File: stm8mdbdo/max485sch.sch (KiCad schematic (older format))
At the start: 1 part, among them U4 MAX485

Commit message: Решена проблемма с библиотекой для конденсаторов. Просто сделал копию папки с именем которое содержится в ошибке.
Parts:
- added R15, R16: 20K, symbol R
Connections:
- wire segments 8 -> 12
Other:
- note added: "Доделать: ставить терминатор, разъем."
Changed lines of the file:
@@
 LIBS:zetex
 LIBS:Zilog
+LIBS:rcl
 LIBS:stm8do-cache
 EELAYER 25 0
@@
 $EndComp
 $Comp
-L GND #PWR085
+L GND #PWR88
 U 1 1 5C686AB8
 P 5650 4600
-F 0 "#PWR085" H 5650 4350 50  0001 C CNN
+F 0 "#PWR88" H 5650 4350 50  0001 C CNN
 F 1 "GND" H 5650 4450 50  0000 C CNN
 F 2 "" H 5650 4600 50  0000 C CNN
@@
 	4650 4150 5050 4150
 $Comp
-L +5V #PWR086
+L +5V #PWR87
 U 1 1 5C6A210B
 P 5650 3250
-F 0 "#PWR086" H 5650 3100 50  0001 C CNN
+F 0 "#PWR87" H 5650 3100 50  0001 C CNN
 F 1 "+5V" H 5650 3390 50  0000 C CNN
 F 2 "" H 5650 3250 50  0000 C CNN
@@
 	4650 3900 4850 3900
 Connection ~ 4850 3900
+$Comp
+L R R15
+U 1 1 5C6B16A1
+P 8150 1850
+F 0 "R15" V 8230 1850 50  0000 C CNN
+F 1 "20K" V 8150 1850 50  0000 C CNN
+F 2 "" V 8080 1850 50  0000 C CNN
+F 3 "" H 8150 1850 50  0000 C CNN
+	1    8150 1850
+	1    0    0    -1
+$EndComp
+$Comp
+L R R16
+U 1 1 5C6B1766
+P 8850 1900
+F 0 "R16" V 8930 1900 50  0000 C CNN
+F 1 "20K" V 8850 1900 50  0000 C CNN
+F 2 "" V 8780 1900 50  0000 C CNN
+F 3 "" H 8850 1900 50  0000 C CNN
+	1    8850 1900
+	1    0    0    -1
+$EndComp
+$Comp
+L +5V #PWR89
+U 1 1 5C6B17A4
+P 8150 1700
+F 0 "#PWR89" H 8150 1550 50  0001 C CNN
+F 1 "+5V" H 8150 1840 50  0000 C CNN
+F 2 "" H 8150 1700 50  0000 C CNN
+F 3 "" H 8150 1700 50  0000 C CNN
+	1    8150 1700
+	1    0    0    -1
+$EndComp
+Text GLabel 8300 2200 2    60   Input ~ 0
+A
+Text GLabel 9000 1600 2    60   Input ~ 0
+B
+$Comp
+L GND #PWR90
+U 1 1 5C6B183A
+P 8850 2050
+F 0 "#PWR90" H 8850 1800 50  0001 C CNN
+F 1 "GND" H 8850 1900 50  0000 C CNN
+F 2 "" H 8850 2050 50  0000 C CNN
+F 3 "" H 8850 2050 50  0000 C CNN
+	1    8850 2050
+	1    0    0    -1
+$EndComp
+Wire Wire Line
+	8150 2000 8150 2200
+Wire Wire Line
+	8150 2200 8300 2200
+Wire Wire Line
+	9000 1600 8850 1600
+Wire Wire Line
+	8850 1600 8850 1750
+Text Notes 4400 1250 0    60   ~ 0
+Доделать: ставить терминатор, разъем.
 $EndSCHEMATC

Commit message: Перевод на новую библиотеку со спасением старых
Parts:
- R15, R16: symbol R -> Device:R
- U6: renamed from U4; symbol MAX485 -> stm8do-rescue:MAX485
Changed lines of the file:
@@
-EESchema Schematic File Version 2
-LIBS:power
-LIBS:device
-LIBS:transistors
-LIBS:conn
-LIBS:linear
-LIBS:regul
-LIBS:74xx
-LIBS:cmos4000
-LIBS:adc-dac
-LIBS:memory
-LIBS:xilinx
-LIBS:microcontrollers
-LIBS:dsp
-LIBS:microchip
-LIBS:analog_switches
-LIBS:motorola
-LIBS:texas
-LIBS:intel
-LIBS:audio
-LIBS:interface
-LIBS:digital-audio
-LIBS:philips
-LIBS:display
-LIBS:cypress
-LIBS:siliconi
-LIBS:opto
-LIBS:atmel
-LIBS:contrib
-LIBS:valves
-LIBS:ac-dc
-LIBS:Altera
-LIBS:analog_devices
-LIBS:Battery_Management
-LIBS:bbd
-LIBS:Bosch
-LIBS:brooktre
-LIBS:Connector
-LIBS:dc-dc
-LIBS:Decawave
-LIBS:Diode
-LIBS:Display
-LIBS:driver_gate
-LIBS:DSP_Microchip_DSPIC33
-LIBS:elec-unifil
-LIBS:ESD_Protection
-LIBS:Espressif
-LIBS:FPGA_Actel
-LIBS:ftdi
-LIBS:gennum
-LIBS:Graphic
-LIBS:hc11
-LIBS:infineon
-LIBS:intersil
-LIBS:ir
-LIBS:Lattice
-LIBS:LED
-LIBS:LEM
-LIBS:Logic_74xgxx
-LIBS:Logic_74xx
-LIBS:Logic_CMOS_4000
-LIBS:Logic_CMOS_IEEE
-LIBS:logic_programmable
-LIBS:Logic_TTL_IEEE
-LIBS:maxim
-LIBS:MCU_Microchip_PIC10
-LIBS:MCU_Microchip_PIC12
-LIBS:MCU_Microchip_PIC16
-LIBS:MCU_Microchip_PIC18
-LIBS:MCU_Microchip_PIC24
-LIBS:MCU_Microchip_PIC32
-LIBS:MCU_NXP_Kinetis
-LIBS:MCU_NXP_LPC
-LIBS:MCU_NXP_S08
-LIBS:MCU_Parallax
-LIBS:MCU_ST_STM8
-LIBS:MCU_ST_STM32
-LIBS:MCU_Texas_MSP430
-LIBS:Mechanical
-LIBS:modules
-LIBS:Motor
-LIBS:motor_drivers
-LIBS:nordicsemi
-LIBS:nxp
-LIBS:onsemi
-LIBS:Oscillators
-LIBS:powerint
-LIBS:Power_Management
-LIBS:pspice
-LIBS:references
-LIBS:Relay
-LIBS:RF_Bluetooth
-LIBS:rfcom
-LIBS:RFSolutions
-LIBS:Sensor_Current
-LIBS:Sensor_Humidity
-LIBS:sensors
-LIBS:silabs
-LIBS:supertex
-LIBS:Switch
-LIBS:Transformer
-LIBS:Transistor
-LIBS:triac_thyristor
-LIBS:Valve
-LIBS:video
-LIBS:wiznet
-LIBS:Worldsemi
-LIBS:Xicor
-LIBS:xilinx-artix7
-LIBS:xilinx-kintex7
-LIBS:xilinx-spartan6
-LIBS:xilinx-virtex5
-LIBS:xilinx-virtex6
-LIBS:xilinx-virtex7
-LIBS:zetex
-LIBS:Zilog
-LIBS:rcl
+EESchema Schematic File Version 4
 LIBS:stm8do-cache
-EELAYER 25 0
+EELAYER 26 0
 EELAYER END
 $Descr A4 11693 8268
@@
 $EndDescr
 $Comp
-L MAX485 U4
+L stm8do-rescue:MAX485 U6
 U 1 1 5C686A16
 P 5650 3900
-F 0 "U4" H 5300 4500 60  0000 C CNN
+F 0 "U6" H 5300 4500 60  0000 C CNN
 F 1 "MAX485" H 5400 4400 60  0000 C CNN
 F 2 "Housings_SOIC:SOIC-8_3.9x4.9mm_Pitch1.27mm" H 5650 3900 60  0001 C CNN
@@
 $EndComp
 $Comp
-L GND #PWR88
+L power:GND #PWR088
 U 1 1 5C686AB8
 P 5650 4600
-F 0 "#PWR88" H 5650 4350 50  0001 C CNN
+F 0 "#PWR088" H 5650 4350 50  0001 C CNN
 F 1 "GND" H 5650 4450 50  0000 C CNN
 F 2 "" H 5650 4600 50  0000 C CNN
@@
 	4650 4150 5050 4150
 $Comp
-L +5V #PWR87
+L power:+5V #PWR087
 U 1 1 5C6A210B
 P 5650 3250
-F 0 "#PWR87" H 5650 3100 50  0001 C CNN
+F 0 "#PWR087" H 5650 3100 50  0001 C CNN
 F 1 "+5V" H 5650 3390 50  0000 C CNN
 F 2 "" H 5650 3250 50  0000 C CNN
@@
 Connection ~ 4850 3900
 $Comp
-L R R15
+L Device:R R15
 U 1 1 5C6B16A1
 P 8150 1850
@@
 $EndComp
 $Comp
-L R R16
+L Device:R R16
 U 1 1 5C6B1766
 P 8850 1900
@@
 $EndComp
 $Comp
-L +5V #PWR89
+L power:+5V #PWR089
 U 1 1 5C6B17A4
 P 8150 1700
-F 0 "#PWR89" H 8150 1550 50  0001 C CNN
+F 0 "#PWR089" H 8150 1550 50  0001 C CNN
 F 1 "+5V" H 8150 1840 50  0000 C CNN
 F 2 "" H 8150 1700 50  0000 C CNN
@@
 B
 $Comp
-L GND #PWR90
+L power:GND #PWR090
 U 1 1 5C6B183A
 P 8850 2050
-F 0 "#PWR90" H 8850 1800 50  0001 C CNN
+F 0 "#PWR090" H 8850 1800 50  0001 C CNN
 F 1 "GND" H 8850 1900 50  0000 C CNN
 F 2 "" H 8850 2050 50  0000 C CNN

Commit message: Auto
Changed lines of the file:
@@
 	5050 4000 4850 4000
 Wire Wire Line
-	4850 4000 4850 3850
+	4850 4000 4850 3900
 Wire Wire Line
 	4850 3850 5050 3850
@@
 Text Notes 4400 1250 0    60   ~ 0
 Доделать: ставить терминатор, разъем.
+Wire Wire Line
+	4850 3900 4850 3850
 $EndSCHEMATC

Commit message: Auto commit date
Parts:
- R15, R16: footprint (none) -> Resistor_SMD:R_0805_2012Metric_Pad1.15x1.40mm_HandSolder
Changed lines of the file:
@@
 F 0 "R15" V 8230 1850 50  0000 C CNN
 F 1 "20K" V 8150 1850 50  0000 C CNN
-F 2 "" V 8080 1850 50  0000 C CNN
+F 2 "Resistor_SMD:R_0805_2012Metric_Pad1.15x1.40mm_HandSolder" V 8080 1850 50  0001 C CNN
 F 3 "" H 8150 1850 50  0000 C CNN
 	1    8150 1850
@@
 F 0 "R16" V 8930 1900 50  0000 C CNN
 F 1 "20K" V 8850 1900 50  0000 C CNN
-F 2 "" V 8780 1900 50  0000 C CNN
+F 2 "Resistor_SMD:R_0805_2012Metric_Pad1.15x1.40mm_HandSolder" V 8780 1900 50  0001 C CNN
 F 3 "" H 8850 1900 50  0000 C CNN
 	1    8850 1900

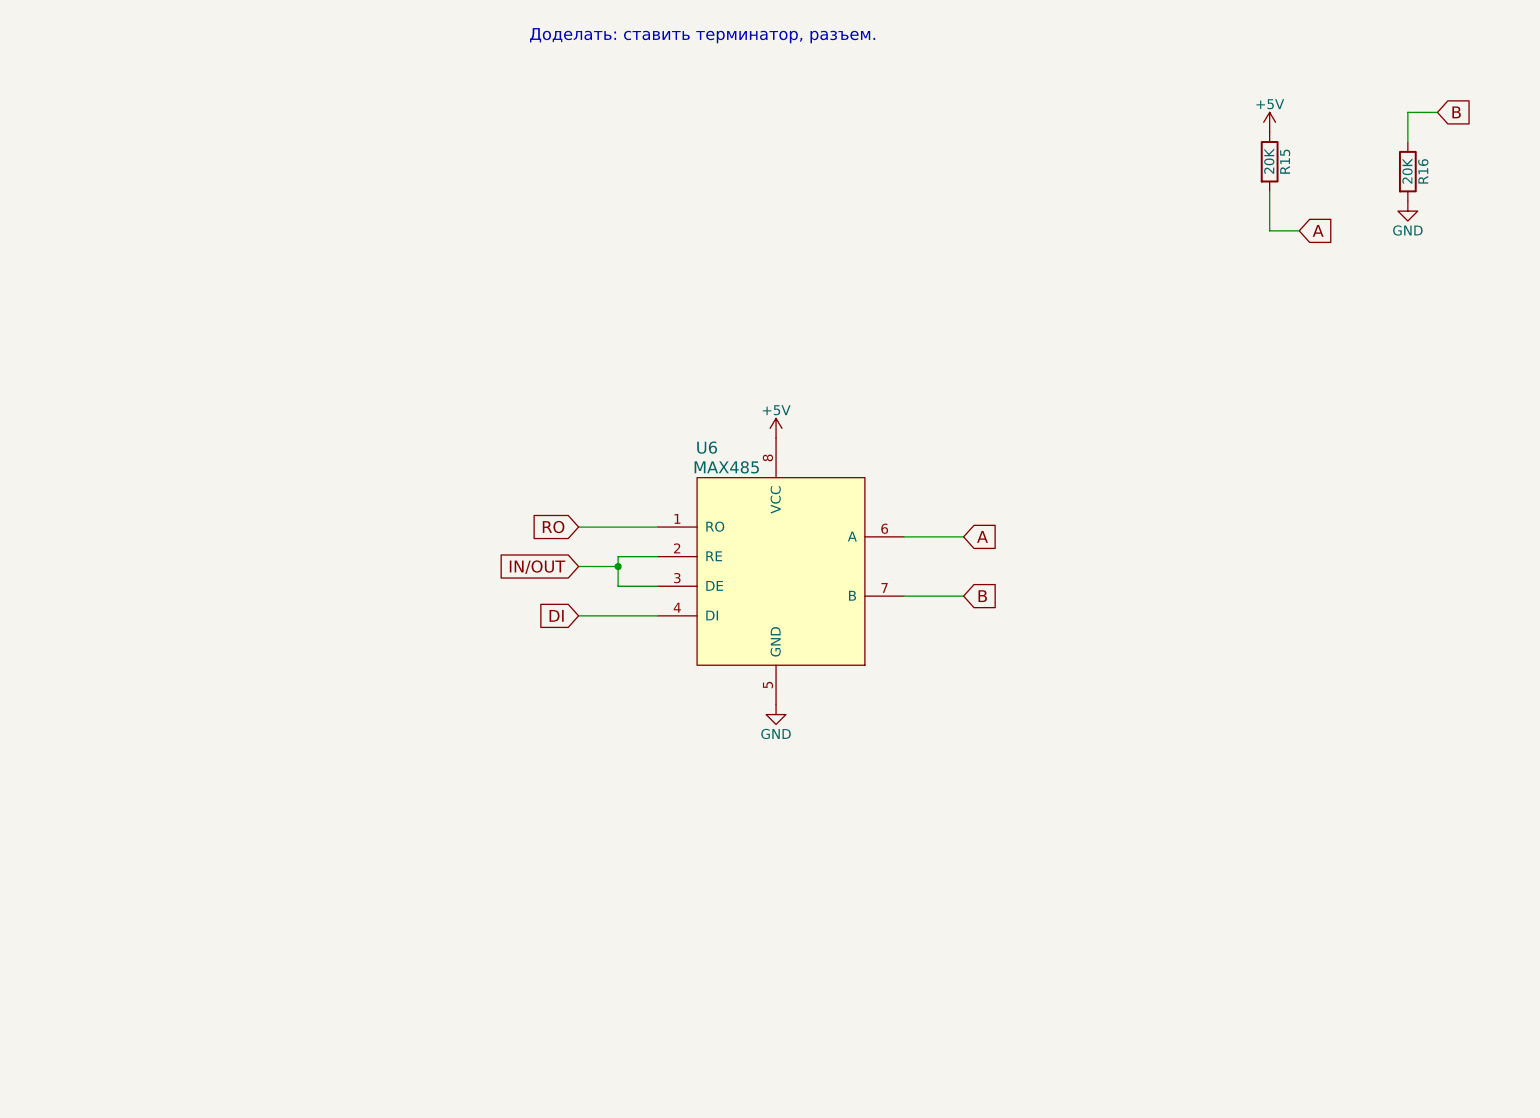
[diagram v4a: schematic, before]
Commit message: Auto commit
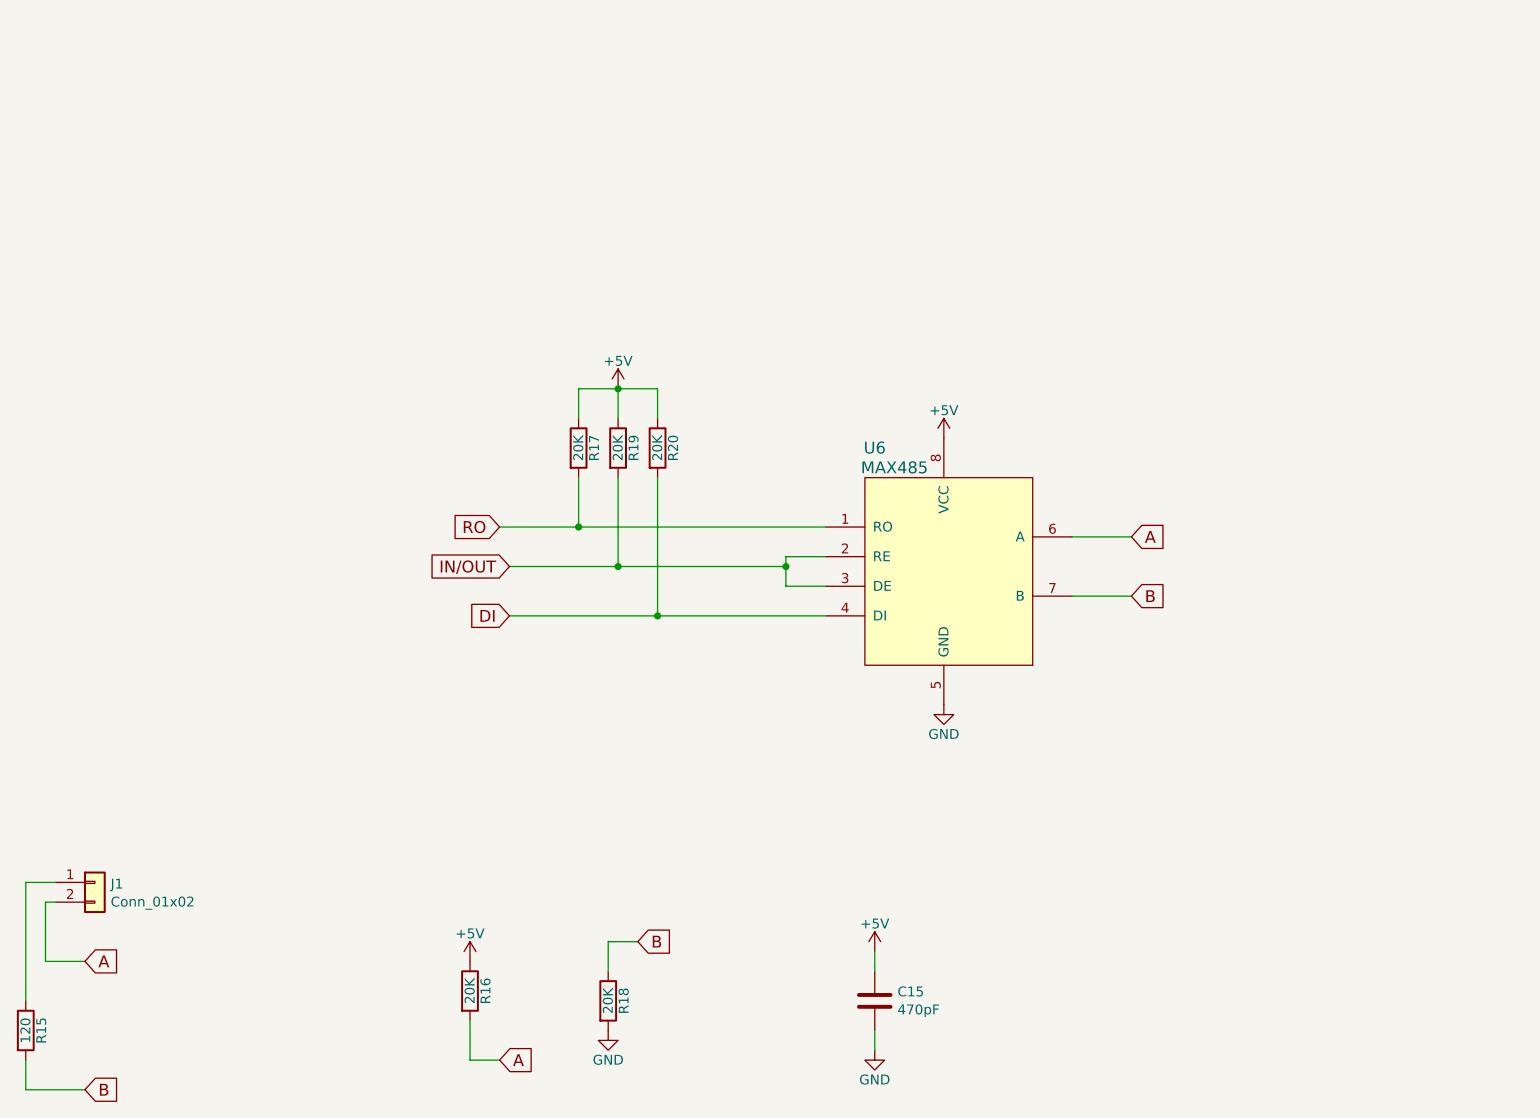
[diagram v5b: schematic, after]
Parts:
- added C15: 470pF, Capacitor_SMD:C_0805_2012Metric_Pad1.15x1.40mm_HandSolder, symbol Device:C
- added J1: Conn_01x02, symbol Connector_Generic:Conn_01x02
- added R15: 120, Resistor_SMD:R_0805_2012Metric_Pad1.15x1.40mm_HandSolder, symbol Device:R
- added R17, R19, R20: 20K, Resistor_SMD:R_0805_2012Metric_Pad1.15x1.40mm_HandSolder, symbol Device:R
- renumbered R15 to R16, R16 to R18
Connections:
- net +5V: now also C15.1, R17.1, R19.1, R20.1
- net A: now also J1.2 (Pin_2)
- net B: now also R15.2
- net DI: now also R20.2
- net GND: now also C15.2
- net IN/OUT: now also R19.2
- net RO: now also R17.2
- new net: J1.1 (Pin_1), R15.1
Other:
- note removed: "Доделать: ставить терминатор, разъем."
- moved on the sheet: R16, R18, U6

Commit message: Auto commit
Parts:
- J1: footprint (none) -> Connector_PinHeader_1.27mm:PinHeader_1x02_P1.27mm_Vertical
- U6: footprint Housings_SOIC:SOIC-8_3.9x4.9mm_Pitch1.27mm -> Package_SO:SOIC-8_3.9x4.9mm_P1.27mm
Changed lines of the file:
@@
 F 0 "U6" H 6150 4500 60  0000 C CNN
 F 1 "MAX485" H 6250 4400 60  0000 C CNN
-F 2 "Housings_SOIC:SOIC-8_3.9x4.9mm_Pitch1.27mm" H 6500 3900 60  0001 C CNN
+F 2 "Package_SO:SOIC-8_3.9x4.9mm_P1.27mm" H 6500 3900 60  0001 C CNN
 F 3 "" H 6500 3900 60  0001 C CNN
 	1    6500 3900
@@
 F 0 "J1" H 2280 5492 50  0000 L CNN
 F 1 "Conn_01x02" H 2280 5401 50  0000 L CNN
-F 2 "" H 2200 5500 50  0001 C CNN
+F 2 "Connector_PinHeader_1.27mm:PinHeader_1x02_P1.27mm_Vertical" H 2200 5500 50  0001 C CNN
 F 3 "~" H 2200 5500 50  0001 C CNN
 	1    2200 5500
